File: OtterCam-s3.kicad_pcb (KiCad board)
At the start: 4 copper layers, 49.7 x 49.7 mm, 167 parts, among them J1 UART, J2 SD, J3 USB, J4 RJ45_Shielded, J5 MIPI, Q1 DTA114YKA, SW1 RST, U1 AllWinner-S3(FBGA-234), U2 AXP209(QFN-48), U3 SY8089AAAC, U4 AP6236, X1 26Mhz TCXO, Y1 32.768kHz, Y2 24MHz

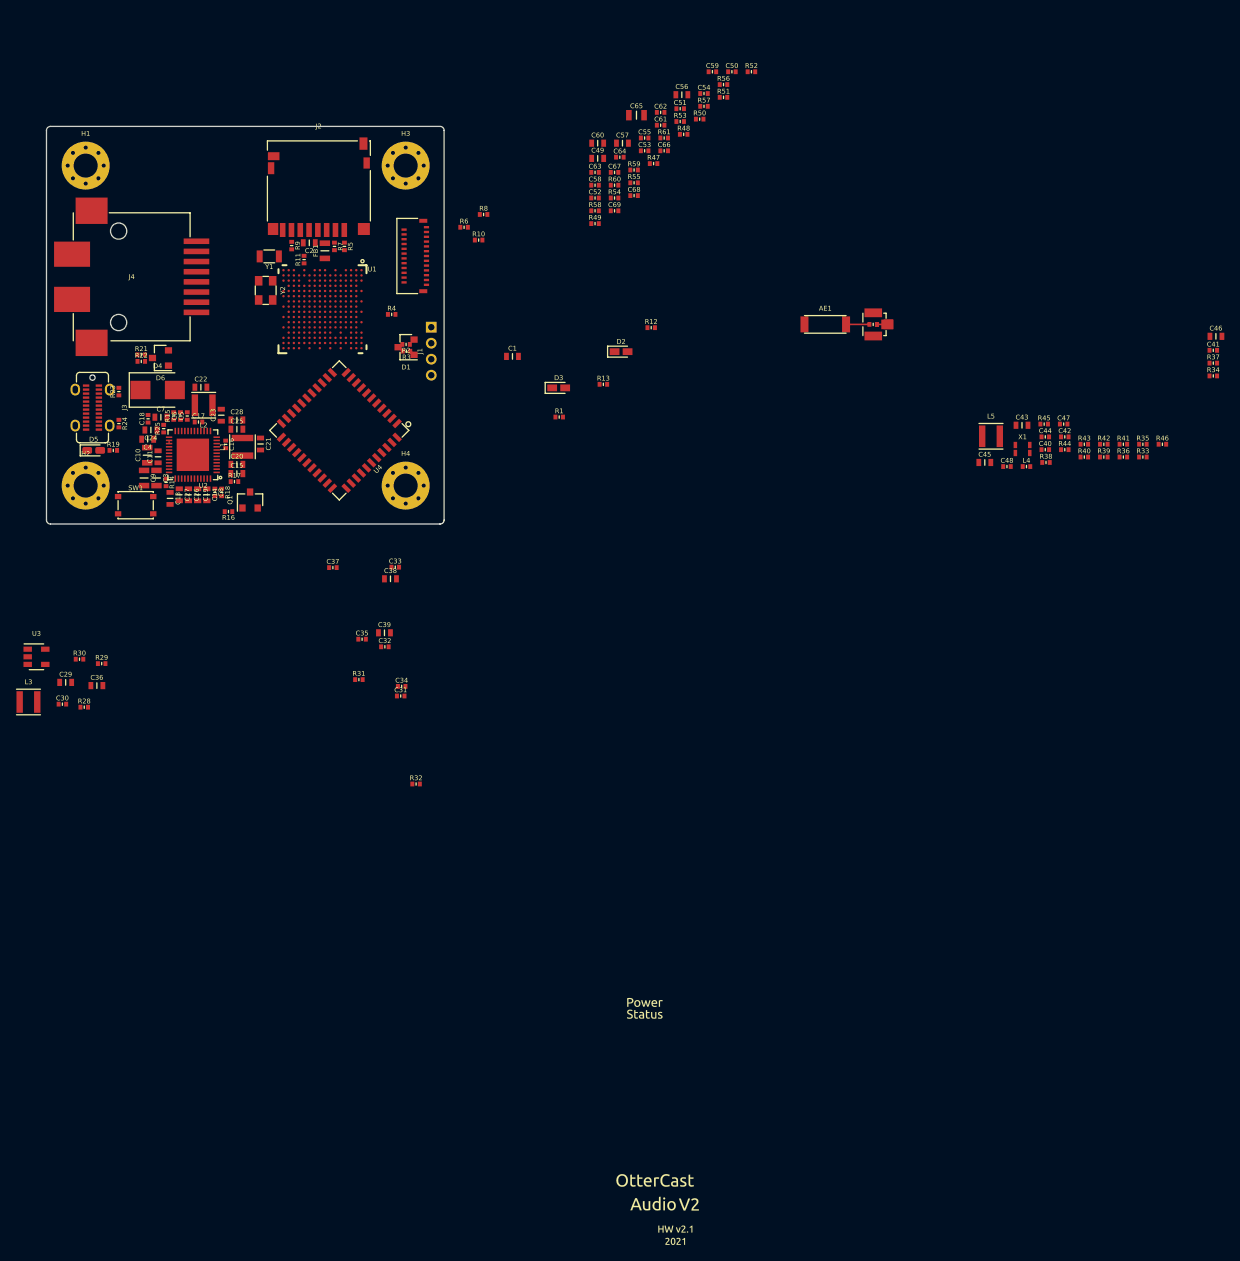
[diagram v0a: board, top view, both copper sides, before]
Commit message: added files
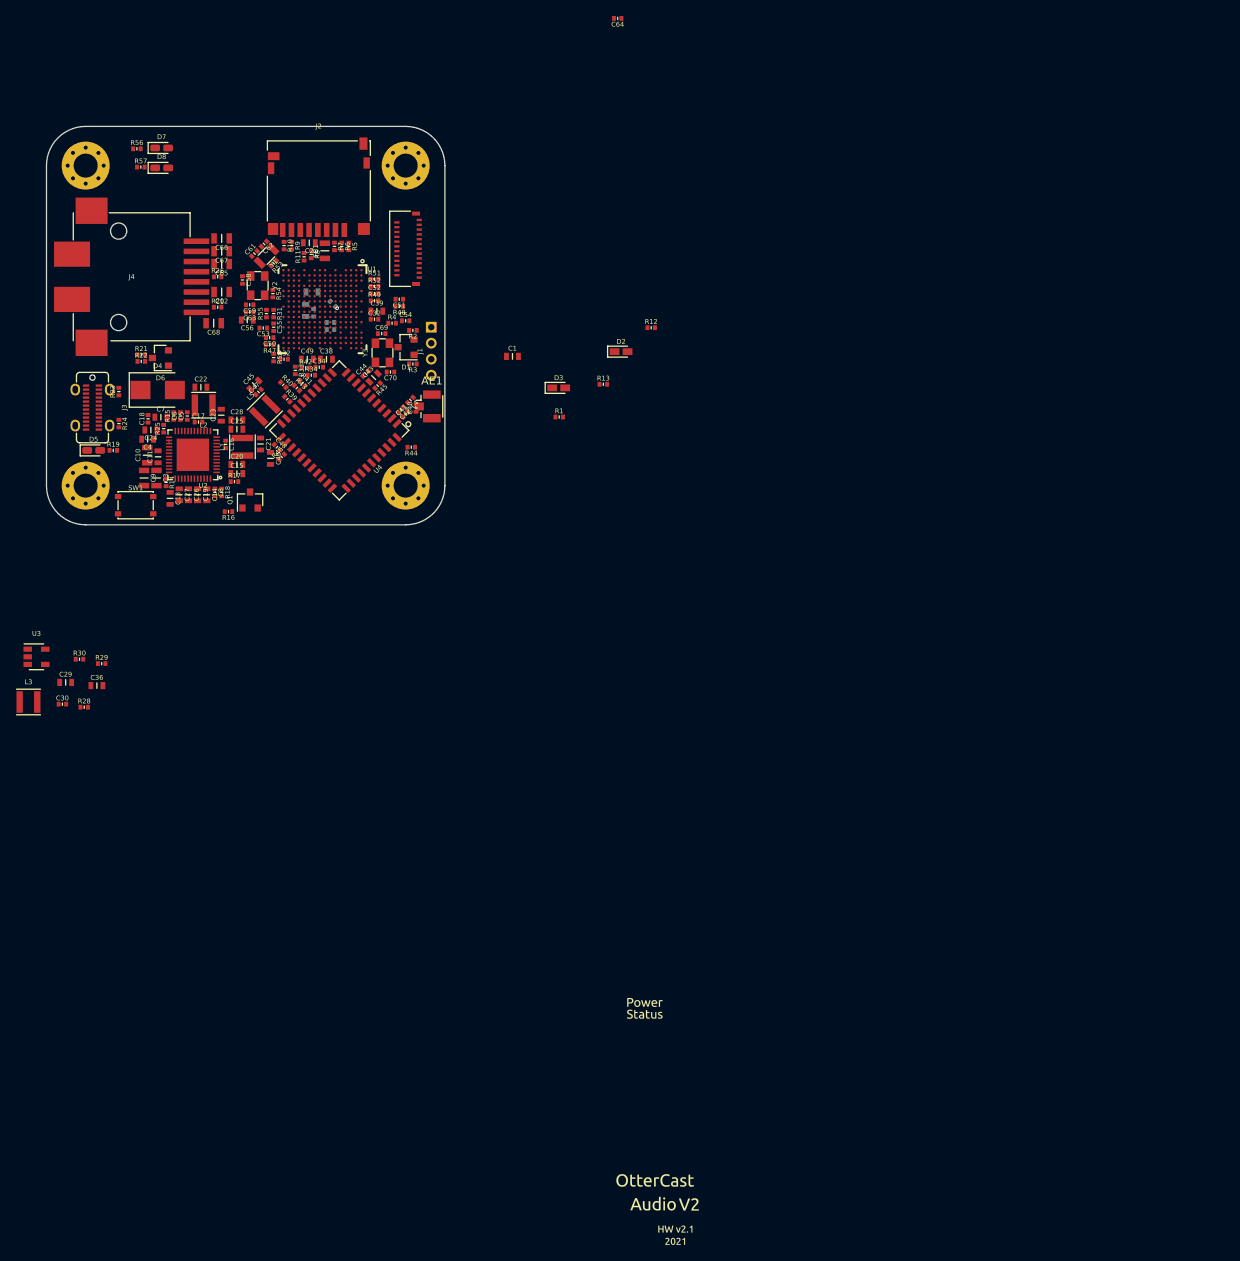
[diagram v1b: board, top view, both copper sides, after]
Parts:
- removed R35, R36, R37, R38: DNP, otter:R_0402
- removed R58, R59, R60, R61: 51, otter:R_0402
- removed X1: 26Mhz TCXO, otter:2016_SMD_CRYSTAL
- added C12: 100n, otter:C_0805, F.Cu at (72.0, 70.8)
- added C70: 18p, otter:C_0402, F.Cu at (93.1, 80.8)
- added D7: YEL, LED_SMD:LED_0603_1608Metric_Castellated, F.Cu at (64.5, 52.8)
- added D8: GRN, LED_SMD:LED_0603_1608Metric_Castellated, F.Cu at (64.5, 55.3)
- added R20: 75, otter:R_0402, F.Cu at (71.5, 72.7)
- added R26: 75, otter:R_0402, F.Cu at (71.5, 68.9)
- added Y3: 26MHz, otter:Oscillator_3225, F.Cu at (92.1, 78.4)
- AE1: footprint otter:KH-5220-A56 -> Connector_Coaxial:U.FL_Hirose_U.FL-R-SMT-1_Vertical
- C31, C33, C35, C37, C57, C60, H1, H2, H3, H4: moved to B.Cu
- C65: value 1n -> 100n
- C66, C67: footprint otter:C_0402 -> otter:C_0805
- C68: value 100n -> 1n; footprint otter:C_0402 -> otter:C_0805
- C69: value 100n -> 18p
- J4: value RJ45_Shielded -> RJ45
- moved C46 119.2 mm to (78.1, 91.6), turned to 270 degrees
- moved R34 112.8 mm to (83.2, 81.2)
- moved R46 110.1 mm to (79.5, 91.4), turned to 45 degrees
- moved R33 106.5 mm to (81.2, 80.6), turned to 270 degrees
- moved R41 102.9 mm to (82.1, 82.2), turned to 315 degrees
- moved R39 102.3 mm to (80.2, 84.2), turned to 315 degrees
- moved C41 101.3 mm to (95.0, 86.1), turned to 45 degrees
- moved C47 100.7 mm to (76.6, 83.3), turned to 45 degrees
- moved R40 100.5 mm to (79.7, 82.4), turned to 315 degrees
- moved R42 100.2 mm to (82.5, 80.3)
- moved R43 98.7 mm to (81.4, 82.8), turned to 315 degrees
- moved C45 91.8 mm to (76.1, 82.4), turned to 45 degrees
- moved C48 91.3 mm to (78.9, 90.2), turned to 315 degrees
- moved L5 90.8 mm to (77.4, 85.6), turned to 45 degrees
- moved C44 85.3 mm to (90.0, 81.0), turned to 45 degrees
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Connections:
- C65 pad 1: Net-(C65-Pad1) -> EPHY_RX_P
- C65 pad 2: GND -> Net-(C65-Pad2)
- C66 pad 1: GND -> EPHY_TX_P
- C67 pad 1: GND -> EPHY_TX_N
- C68 pad 1: GND -> Net-(C68-Pad1)
- C68 pad 2: Net-(C68-Pad2) -> GND
- C69 pad 1: GND -> Net-(C69-Pad1)
- C69 pad 2: Net-(C69-Pad2) -> GND
- J4 pad 1: Net-(J4-Pad1) -> Net-(C66-Pad2)
- J4 pad 2: Net-(J4-Pad2) -> Net-(C67-Pad2)
- J4 pad 3: Net-(J4-Pad3) -> Net-(C65-Pad2)
- J4 pad 5: Net-(J4-Pad5) -> Net-(J4-Pad4)
- J4 pad 8: Net-(J4-Pad8) -> Net-(J4-Pad7)
- U4 pad 11: Net-(U4-Pad11) -> Net-(C69-Pad1)
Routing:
- net VCC-DDR: track 0.00 -> 0.77 mm, vias 0 -> 1
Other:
- board size 49.7 x 49.7 mm -> 49.8 x 49.8 mm
